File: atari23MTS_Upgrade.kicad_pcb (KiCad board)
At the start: 2 copper layers, 98 x 119.5 mm, 83 parts, among them J1 Conn_01x02, J2 Conn_01x02, J3 Conn_01x02, J4 Conn_01x02, J5 Conn_01x02, J6 Conn_01x02, J7 Conn_01x02, J8 Conn_01x02, J9 Micro_SD_Card_Det, P1 CONN_01X01, P2 CONN_01X01, P3 CONN_01X01, P4 CONN_01X01, P5 CONN_01X01, P6 CONN_01X01, P7 CONN_01X01, P8 CONN_01X01, SW1 SW_Push, U1 NCP1117ST33T3G, U10 74LVC2G32, U11 74LVC2G08, U12 74LVC2G74, U13 STM32F407VETx, U2 TXB0108-PW, U3 TXB0108-PW, U4 TXB0108-PW, U5 TXB0108-PW, U6 TXB0108-PW, U7 ISSI61WV5128BL, U8 ISSI61WV5128BL, U9 74HCT04

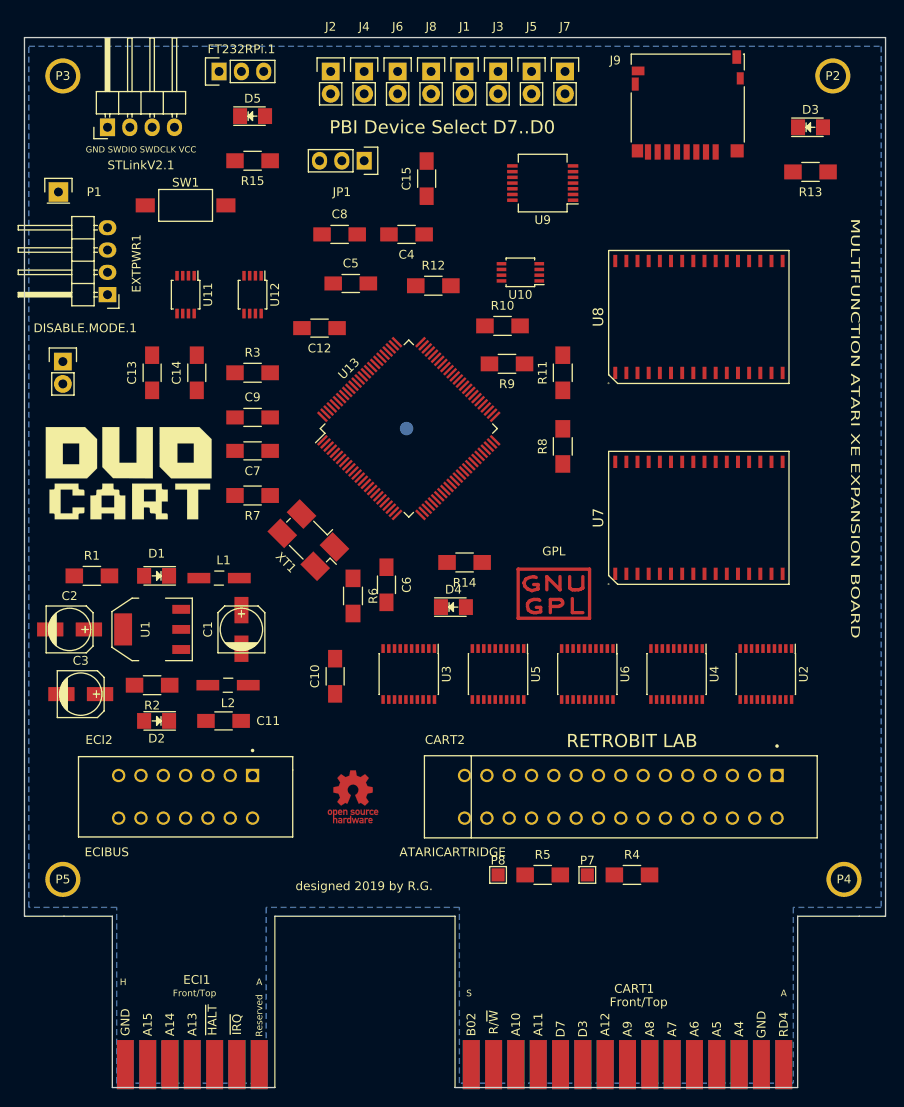
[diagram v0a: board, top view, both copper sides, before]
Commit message: Upgraded after last routing
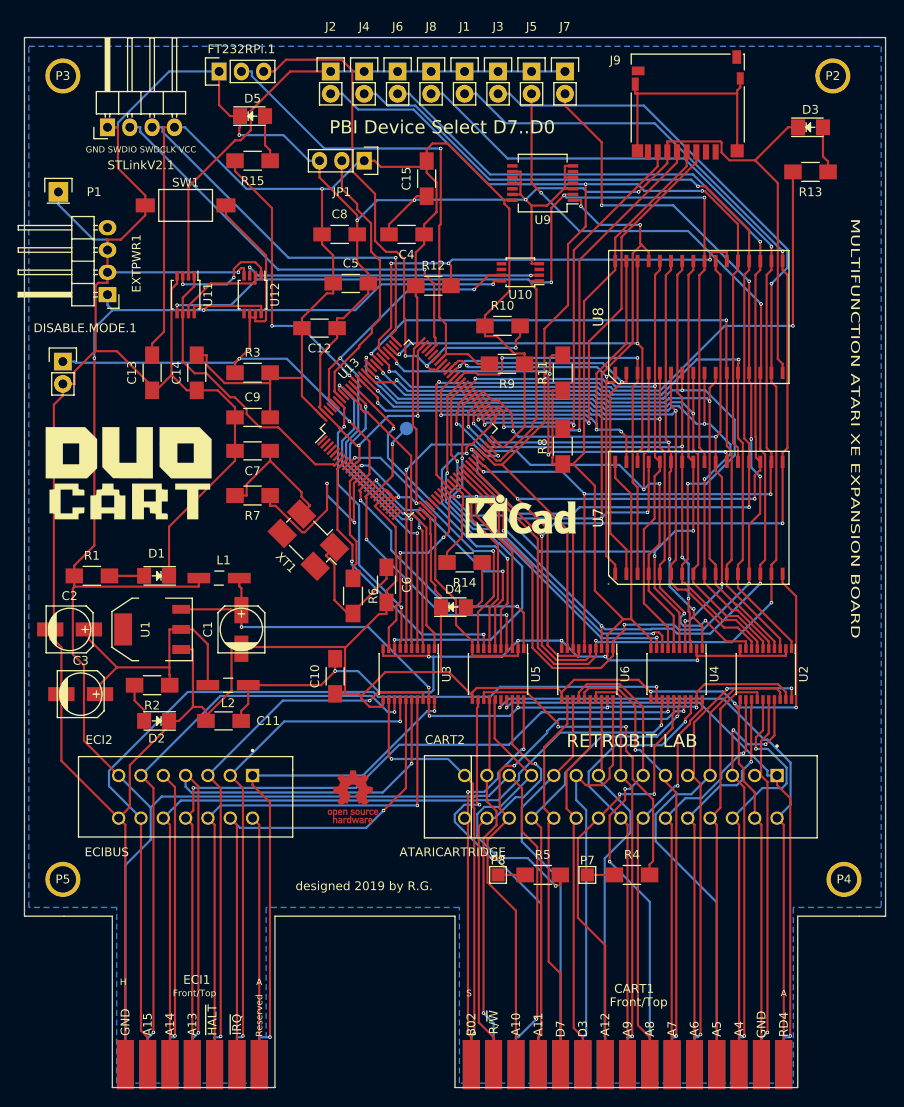
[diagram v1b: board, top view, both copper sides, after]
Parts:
- removed GPL: Symbol_GNU-GPL_CopperTop_Small, Symbol:Symbol_GNU-GPL_CopperTop_Small
- added Kicad: KiCad-Logo_5mm_SilkScreen, Symbol:KiCad-Logo_5mm_SilkScreen, F.Cu at (155.0, 74.0)
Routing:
- net GND: track 0.00 -> 629.3 mm, vias 0 -> 11
- net VCC3V3: track 0.00 -> 429.5 mm, vias 0 -> 10
- net +5VDC: track 0.00 -> 243.0 mm, vias 0 -> 4
- net mD7: track 0.00 -> 142.6 mm, vias 0 -> 2
- net mD2: track 0.00 -> 136.9 mm, vias 0 -> 3
- net mD6: track 0.00 -> 134.9 mm, vias 0 -> 4
- net mD5: track 0.00 -> 134.8 mm, vias 0 -> 3
- net mD3: track 0.00 -> 134.2 mm, vias 0 -> 3
- net mD4: track 0.00 -> 127.9 mm, vias 0 -> 4
- net mD0: track 0.00 -> 124.7 mm, vias 0 -> 6
- net mD1: track 0.00 -> 122.5 mm, vias 0 -> 5
- net A15: track 0.00 -> 103.5 mm, vias 0 -> 1
- net mW/~R: track 0.00 -> 103.1 mm, vias 0 -> 4
- net mR/~W: track 0.00 -> 96.3 mm, vias 0 -> 6
- net A14: track 0.00 -> 92.8 mm, vias 0 -> 1
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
